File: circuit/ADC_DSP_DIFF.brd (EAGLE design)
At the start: 50 x 76.8 mm, 79 parts, among them IC1 REG1117, IC3 STM32F40XRXT6, IC4 CS4272, Q1 8MHz, Q2 24.576MHz

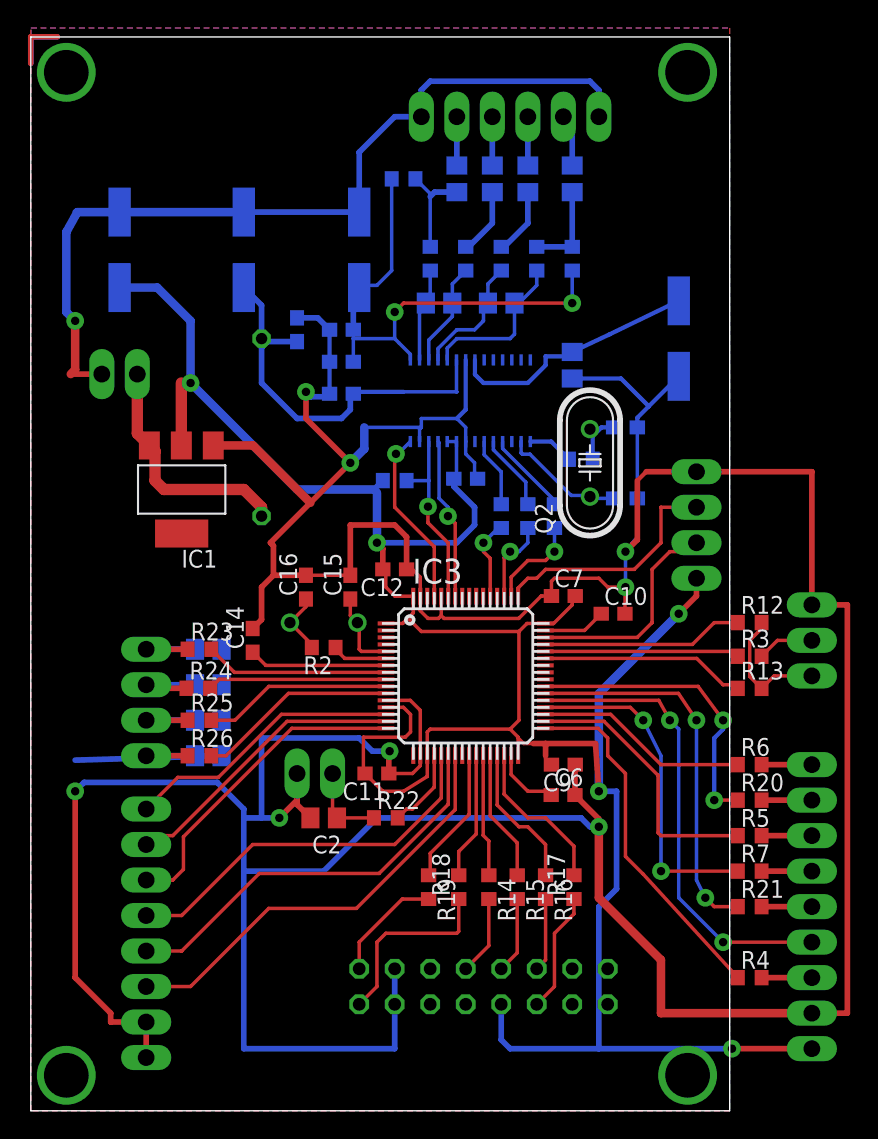
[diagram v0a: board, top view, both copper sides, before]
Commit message: - вроде все линии переразвели
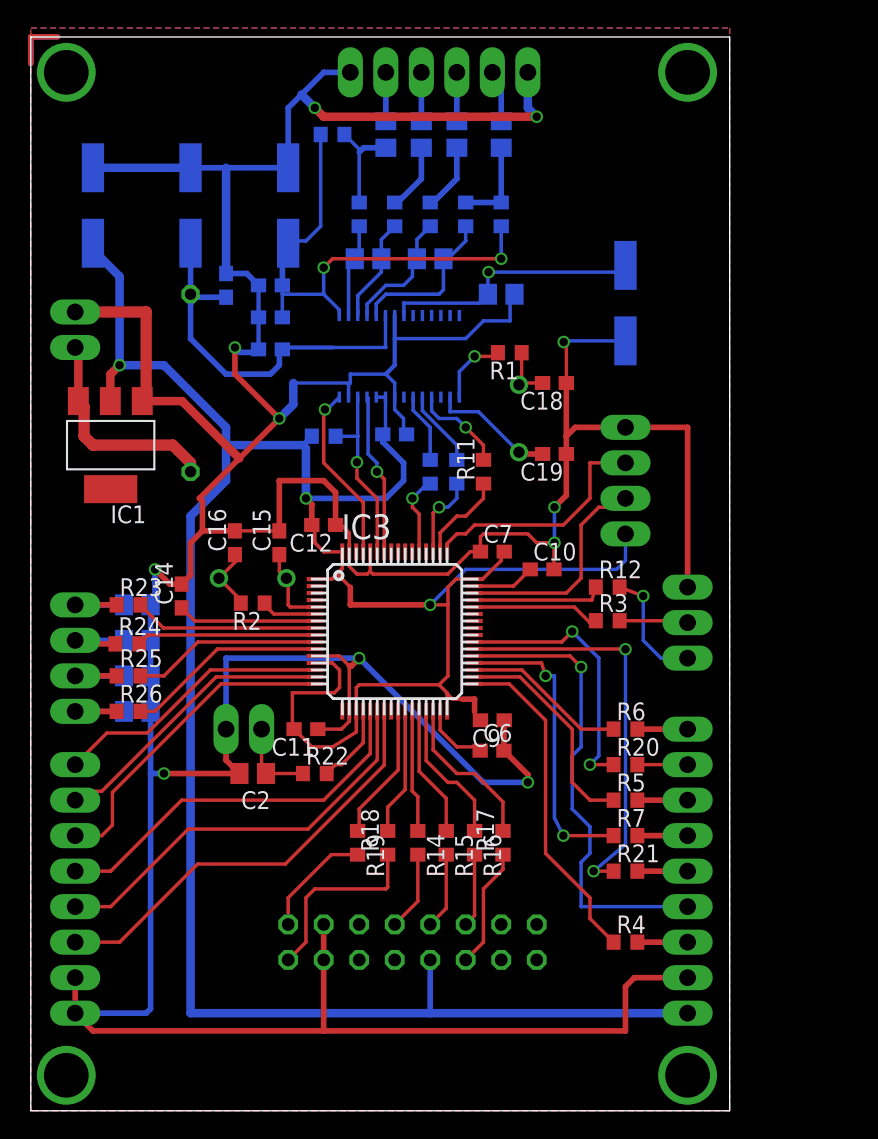
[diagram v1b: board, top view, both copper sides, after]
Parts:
- removed R13: 1K5(infinity), rcl:R0603
- moved R12 10.5 mm to (41.3, 37.5)
- moved R3 10.5 mm to (41.3, 35.1)
- moved LCD 9.25 mm to (47.0, 17.1)
- moved R20 9.25 mm to (42.5, 24.8)
- moved R21 9.25 mm to (42.5, 17.1)
- moved R4 9.25 mm to (42.5, 12.1)
- moved R5 9.25 mm to (42.5, 22.2)
- moved R6 9.25 mm to (42.5, 27.3)
- moved R7 9.25 mm to (42.5, 19.7)
- moved R1 9.16 mm to (34.3, 54.2), flipped to the top, turned to 180 degrees
- moved USB 8.98 mm to (47.0, 34.9)
- moved C24 7.18 mm to (33.7, 58.4), turned to 180 degrees
- moved Q2 5.99 mm to (34.9, 49.5), flipped to the bottom
- moved C26 5.99 mm to (17.1, 54.5)
- moved C27 5.99 mm to (28.6, 61.0)
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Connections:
- removed net PA10(USB_ON): IC3.43, R13.1
- net D+: no longer R13.2
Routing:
- net GND: track 418.8 -> 367.5 mm, vias 9 -> 11
- net +3V3: track 182.1 -> 208.6 mm, vias 5 -> 3
- net PA10(USB_ON): track 14.7 -> 0.00 mm
- net USB_DP: track 14.4 -> 9.37 mm
- net USB_DM: track 13.9 -> 9.21 mm
- net PB13(TFT_SCK): track 19.6 -> 15.8 mm
- net PB14(TFT_MISO): track 15.3 -> 11.7 mm
- net PB15(TFT_MOSI): track 24.0 -> 21.6 mm
- net PC8(TFT_LED): track 21.6 -> 19.6 mm
- net PC7(TFT_D_C): track 27.3 -> 29.2 mm
- net N$17: track 3.29 -> 5.15 mm, vias 0 -> 1
- net +5V: track 17.2 -> 15.7 mm
- net PB12(TFT_CS): track 25.6 -> 24.1 mm
- net D-: track 4.07 -> 4.92 mm
- net N$12: track 18.0 -> 18.8 mm, vias 0 -> 1
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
